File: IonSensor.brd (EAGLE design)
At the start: 50.8 x 22.9 mm, 20 parts, among them IC1 QUAD_OPAMPD, IC2 QUAD_OPAMPD, IC3 QUAD_OPAMPD, X1 JST-XH-04-PIN-LONG-PAD

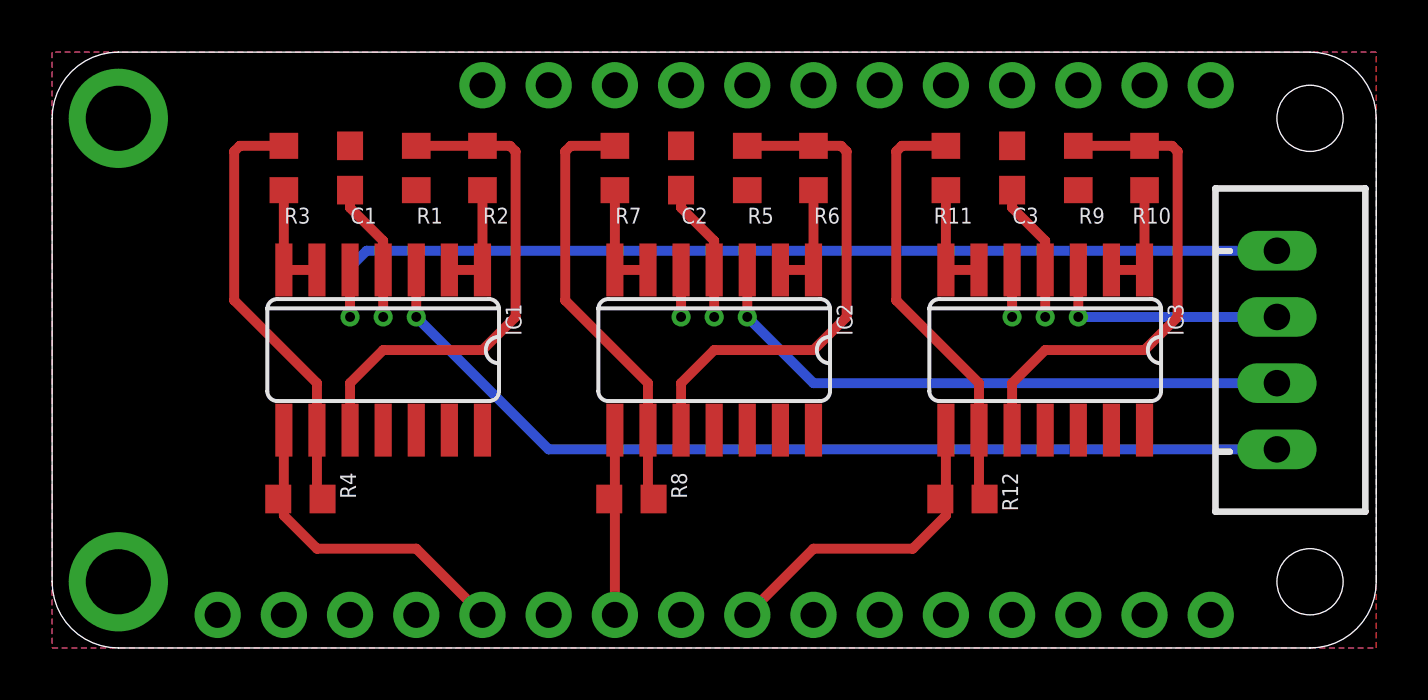
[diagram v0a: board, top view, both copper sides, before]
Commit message: Switch to 2 channel opamp
Switched to 2 channel opamp instead of quad opamp.
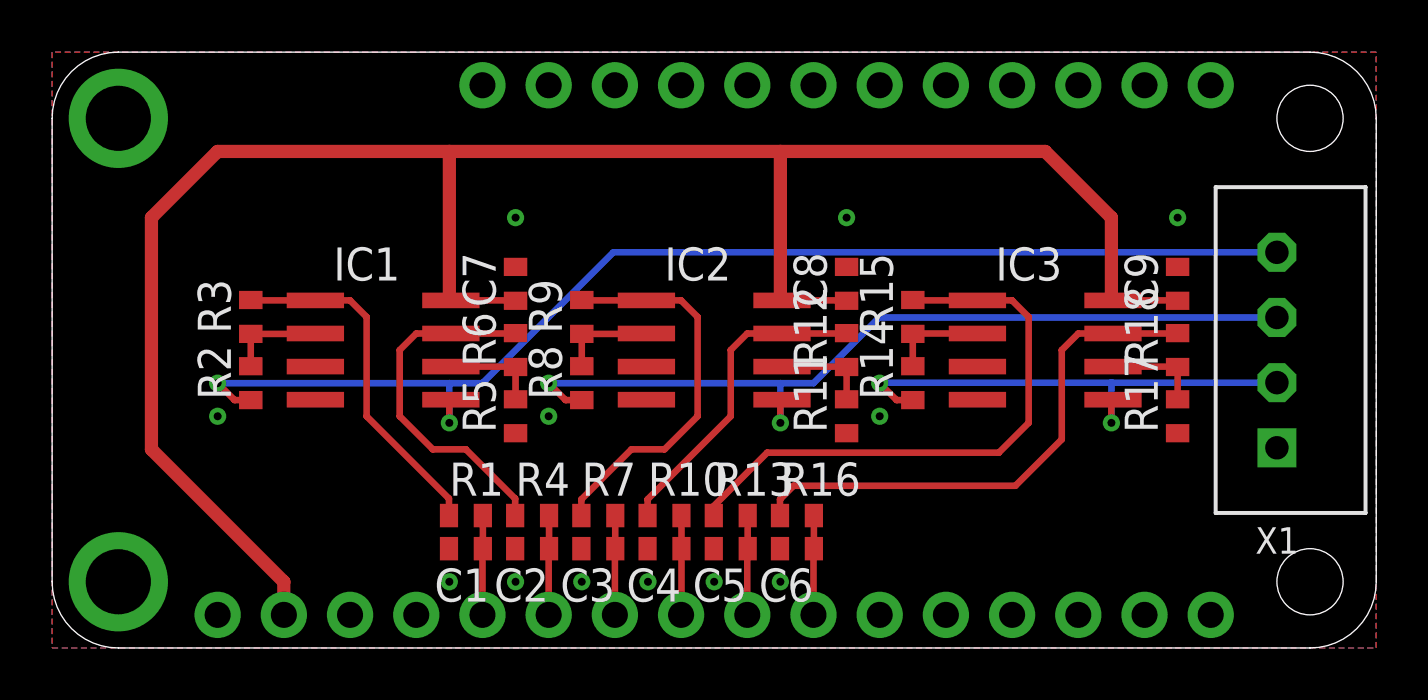
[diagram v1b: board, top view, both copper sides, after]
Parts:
- added C4, C5, C6, C7, C8, C9: 0.1uF, adafruit:C0402
- added R13, R16: 1M, adafruit:R0402
- added R14, R17, R18: 10k, adafruit:R0402
- added R15: 20k, adafruit:R0402
- C1, C2, C3: device adafruit:C0603 -> adafruit:C0402
- IC1, IC2, IC3: value QUAD_OPAMPD -> LM358D; device adafruit:SO14 -> linear:SO08
- R1, R4: value 100k -> 1M; device adafruit:R0603 -> adafruit:R0402
- R10, R7: value 10k -> 1M; device adafruit:R0603 -> adafruit:R0402
- R11, R2, R6: device adafruit:R0603 -> adafruit:R0402
- R12, R5, R8: value 100k -> 10k; device adafruit:R0603 -> adafruit:R0402
- R3: value 10k -> 20k; device adafruit:R0603 -> adafruit:R0402
- R9: value 100k -> 20k; device adafruit:R0603 -> adafruit:R0402
- X1: value JST-XH-04-PIN-LONG-PAD -> B4B-XH-2; device Rembrandt Electronics - JST XH Connectors v1-0:JST-XH-04-PACKAGE-LONG-PAD -> con-JST XH:B4B-XH-A
- moved R10 22.7 mm to (23.5, 5.08), turned to 0 degrees
- moved C3 21.6 mm to (21.0, 3.81), turned to 180 degrees
- moved R9 19.9 mm to (20.3, 12.7)
- moved C2 15.7 mm to (18.4, 3.81), turned to 180 degrees
- moved C1 15.3 mm to (15.9, 3.81), turned to 180 degrees
- moved R1 13.5 mm to (15.9, 5.08), turned to 0 degrees
- moved R6 13.4 mm to (17.8, 11.4)
- moved R7 13.4 mm to (21.0, 5.08), turned to 0 degrees
- moved R5 13.0 mm to (17.8, 8.89)
- moved R2 12.1 mm to (7.62, 10.2)
- moved R11 10.3 mm to (30.5, 8.89)
- moved R4 8.91 mm to (18.4, 5.08), turned to 0 degrees
- moved R12 7.24 mm to (30.5, 11.4), turned to 90 degrees
- moved R3 5.85 mm to (7.62, 12.7)
- moved R8 4.84 mm to (20.3, 10.2), turned to 90 degrees
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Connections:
- removed net N$13: IC3.10, R10.2, R9.2
- removed net N$14: IC3.9, R11.2, R12.1
- removed net REF: IC1.5, IC2.5, IC3.5, X1.1
- new net A1: C2.1, MS1.6, R4.2
- new net A3: C4.1, MS1.8, R10.2
- new net A5: C6.1, MS1.10, R16.2
- new net N$10: IC3.1, R13.1, R15.2
- new net N$5: IC2.2, R8.2, R9.1
- net +3V3: now also C7.1, C8.1, C9.1, IC1.8, IC2.8, IC3.8; no longer C1.1, C2.1, C3.1, IC1.4, IC2.4, IC3.4
- net A0: now also C1.1, R1.2; no longer IC1.8, R4.2
- net A2: now also C3.1, R7.2; no longer IC2.8, R8.2
- net A4: now also C5.1, R13.2; no longer IC3.8, R12.2
- net CH0: now also IC1.5, R2.1; no longer IC1.3
- net CH1: now also IC2.5, R8.1; no longer IC2.3
- net CH2: now also IC3.5, R14.1; no longer IC3.3
- net GND: now also C4.2, C5.2, C6.2, C7.2, C8.2, C9.2, IC1.3, IC1.4, IC2.3, IC2.4, IC3.3, IC3.4, R11.1, R17.1, X1.1; no longer IC1.11, IC2.11, IC3.11, R1.1, R9.1
- net N$1: now also R2.2, R3.1; no longer IC1.1, R2.1
- net N$11: now also IC3.6, R17.2, R18.1; no longer IC3.1, IC3.2, R10.1
- net N$12: now also R16.1, R18.2; no longer IC3.6, R11.1
- net N$2: now also IC1.6, R5.2, R6.1; no longer IC1.10, R1.2, R2.2
- net N$3: now also IC1.1, R1.1, R3.2; no longer IC1.6, IC1.7, R3.1
- net N$4: now also IC1.7, R6.2; no longer IC1.9, R3.2
- net N$6: now also R7.1, R9.2; no longer IC2.2, R6.1
- net N$7: now also R11.2, R12.1; no longer IC2.7, R7.1
- net N$8: now also IC2.7, R10.1, R12.2; no longer IC2.10, R5.2, R6.2
- net N$9: now also IC3.2, R14.2, R15.1; no longer IC2.9, R7.2, R8.1
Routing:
- net +3V3: track 16.2 -> 78.4 mm, vias 3 -> 0
- net REF: track 48.2 -> 0.00 mm, vias 3 -> 0
- net N$10: track 0.00 -> 22.5 mm
- net N$13: track 19.5 -> 0.00 mm
- net N$14: track 16.7 -> 0.00 mm
- net N$12: track 4.33 -> 20.5 mm
- net N$2: track 19.5 -> 3.73 mm
- net N$9: track 16.7 -> 3.73 mm
- net N$6: track 4.33 -> 14.9 mm
- net CH2: track 9.42 -> 19.2 mm, vias 1 -> 2
- net CH1: track 23.2 -> 33.0 mm, vias 1 -> 2
- net CH0: track 36.9 -> 46.7 mm, vias 1 -> 2
- net N$3: track 4.33 -> 13.6 mm
- net A0: track 12.7 -> 3.82 mm
- net A4: track 12.7 -> 3.82 mm
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- added copper zone on layer 16, net GND
- removed copper zone on layer 16, net +3V3
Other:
- board text added: "Rev. D"

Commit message: Revert "Switch to 2 channel opamp"
This reverts commit d2c6276b5e9005aaa4bb267ec01d57cf95291150.
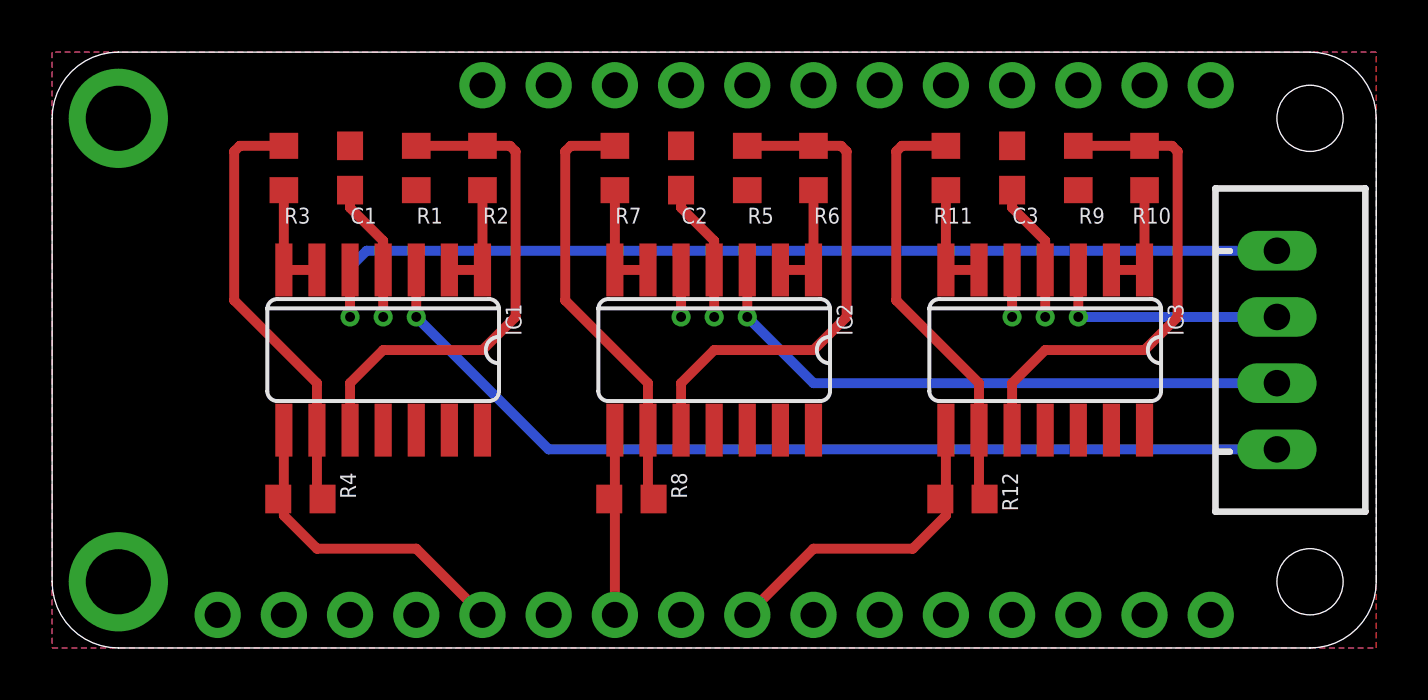
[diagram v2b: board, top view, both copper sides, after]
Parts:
- removed C4, C5, C6, C7, C8, C9: 0.1uF, adafruit:C0402
- removed R13, R16: 1M, adafruit:R0402
- removed R14, R17, R18: 10k, adafruit:R0402
- removed R15: 20k, adafruit:R0402
- C1, C2, C3: device adafruit:C0402 -> adafruit:C0603
- IC1, IC2, IC3: value LM358D -> QUAD_OPAMPD; device linear:SO08 -> adafruit:SO14
- R1, R4: value 1M -> 100k; device adafruit:R0402 -> adafruit:R0603
- R10, R7: value 1M -> 10k; device adafruit:R0402 -> adafruit:R0603
- R11, R2, R6: device adafruit:R0402 -> adafruit:R0603
- R12, R5, R8: value 10k -> 100k; device adafruit:R0402 -> adafruit:R0603
- R3: value 20k -> 10k; device adafruit:R0402 -> adafruit:R0603
- R9: value 20k -> 100k; device adafruit:R0402 -> adafruit:R0603
- X1: value B4B-XH-2 -> JST-XH-04-PIN-LONG-PAD; device con-JST XH:B4B-XH-A -> Rembrandt Electronics - JST XH Connectors v1-0:JST-XH-04-PACKAGE-LONG-PAD
- moved R10 22.7 mm to (41.9, 18.4), turned to 90 degrees
- moved C3 21.6 mm to (36.8, 18.4), turned to 90 degrees
- moved R9 19.9 mm to (39.4, 18.4)
- moved C2 15.7 mm to (24.1, 18.4), turned to 90 degrees
- moved C1 15.3 mm to (11.4, 18.4), turned to 90 degrees
- moved R1 13.5 mm to (14.0, 18.4), turned to 90 degrees
- moved R6 13.4 mm to (29.2, 18.4)
- moved R7 13.4 mm to (21.6, 18.4), turned to 90 degrees
- moved R5 13.0 mm to (26.7, 18.4)
- moved R2 12.1 mm to (16.5, 18.4)
- moved R11 10.3 mm to (34.3, 18.4)
- moved R4 8.91 mm to (9.53, 5.71), turned to 180 degrees
- moved R12 7.24 mm to (34.9, 5.71), turned to 180 degrees
- moved R3 5.85 mm to (8.89, 18.4)
- moved R8 4.84 mm to (22.2, 5.71), turned to 180 degrees
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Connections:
- removed net A1: C2.1, MS1.6, R4.2
- removed net A3: C4.1, MS1.8, R10.2
- removed net A5: C6.1, MS1.10, R16.2
- removed net N$10: IC3.1, R13.1, R15.2
- removed net N$5: IC2.2, R8.2, R9.1
- new net N$13: IC3.10, R10.2, R9.2
- new net N$14: IC3.9, R11.2, R12.1
- new net REF: IC1.5, IC2.5, IC3.5, X1.1
- net +3V3: now also C1.1, C2.1, C3.1, IC1.4, IC2.4, IC3.4; no longer C7.1, C8.1, C9.1, IC1.8, IC2.8, IC3.8
- net A0: now also IC1.8, R4.2; no longer C1.1, R1.2
- net A2: now also IC2.8, R8.2; no longer C3.1, R7.2
- net A4: now also IC3.8, R12.2; no longer C5.1, R13.2
- net CH0: now also IC1.3; no longer IC1.5, R2.1
- net CH1: now also IC2.3; no longer IC2.5, R8.1
- net CH2: now also IC3.3; no longer IC3.5, R14.1
- net GND: now also IC1.11, IC2.11, IC3.11, R1.1, R9.1; no longer C4.2, C5.2, C6.2, C7.2, C8.2, C9.2, IC1.3, IC1.4, IC2.3, IC2.4, IC3.3, IC3.4, R11.1, R17.1, X1.1
- net N$1: now also IC1.1, R2.1; no longer R2.2, R3.1
- net N$11: now also IC3.1, IC3.2, R10.1; no longer IC3.6, R17.2, R18.1
- net N$12: now also IC3.6, R11.1; no longer R16.1, R18.2
- net N$2: now also IC1.10, R1.2, R2.2; no longer IC1.6, R5.2, R6.1
- net N$3: now also IC1.6, IC1.7, R3.1; no longer IC1.1, R1.1, R3.2
- net N$4: now also IC1.9, R3.2; no longer IC1.7, R6.2
- net N$6: now also IC2.2, R6.1; no longer R7.1, R9.2
- net N$7: now also IC2.7, R7.1; no longer R11.2, R12.1
- net N$8: now also IC2.10, R5.2, R6.2; no longer IC2.7, R10.1, R12.2
- net N$9: now also IC2.9, R7.2, R8.1; no longer IC3.2, R14.2, R15.1
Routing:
- net +3V3: track 78.4 -> 16.2 mm, vias 0 -> 3
- net REF: track 0.00 -> 48.2 mm, vias 0 -> 3
- net N$10: track 22.5 -> 0.00 mm
- net N$13: track 0.00 -> 19.5 mm
- net N$14: track 0.00 -> 16.7 mm
- net N$12: track 20.5 -> 4.33 mm
- net N$2: track 3.73 -> 19.5 mm
- net N$9: track 3.73 -> 16.7 mm
- net N$6: track 14.9 -> 4.33 mm
- net CH2: track 19.2 -> 9.42 mm, vias 2 -> 1
- net CH1: track 33.0 -> 23.2 mm, vias 2 -> 1
- net CH0: track 46.7 -> 36.9 mm, vias 2 -> 1
- net N$3: track 13.6 -> 4.33 mm
- net A0: track 3.82 -> 12.7 mm
- net A4: track 3.82 -> 12.7 mm
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- added copper zone on layer 16, net +3V3
- removed copper zone on layer 16, net GND
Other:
- board text removed: "Rev. D"

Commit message: Rev. D
Upgrade to Rev. D, no connector
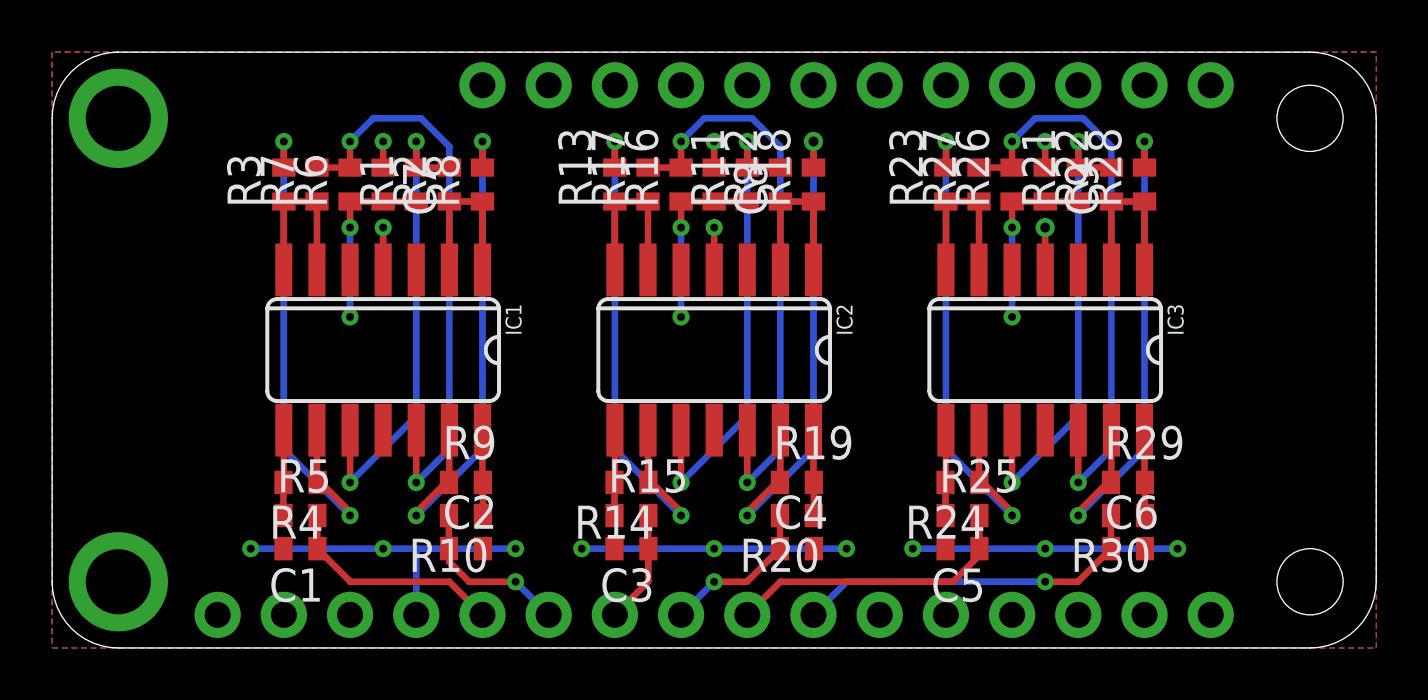
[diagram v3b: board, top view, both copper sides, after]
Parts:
- removed X1: JST-XH-04-PIN-LONG-PAD, Rembrandt Electronics - JST XH Connectors v1-0:JST-XH-04-PACKAGE-LONG-PAD
- added C4, C5, C6, C7, C8, C9: 0.1uF, adafruit:C0402
- added R13, R17, R18, R22, R23, R27, R28: 10k, adafruit:R0402
- added R14, R16, R19, R21, R24, R26, R29: 100k, adafruit:R0402
- added R15, R20, R25, R30: 1M, adafruit:R0402
- C1, C2, C3: device adafruit:C0603 -> adafruit:C0402
- R1, R2, R3, R4, R7, R9: device adafruit:R0603 -> adafruit:R0402
- R10: value 10k -> 1M; device adafruit:R0603 -> adafruit:R0402
- R11, R6: value 10k -> 100k; device adafruit:R0603 -> adafruit:R0402
- R12, R8: value 100k -> 10k; device adafruit:R0603 -> adafruit:R0402
- R5: value 100k -> 1M; device adafruit:R0603 -> adafruit:R0402
- moved R10 29.3 mm to (15.9, 5.08), turned to 180 degrees
- moved R9 26.4 mm to (15.9, 6.35), turned to 0 degrees
- moved R5 21.7 mm to (9.53, 5.08), turned to 0 degrees
- moved C3 20.7 mm to (22.2, 3.81), turned to 180 degrees
- moved R6 17.8 mm to (11.4, 17.8)
- moved C2 16.8 mm to (15.9, 3.81), turned to 0 degrees
- moved C1 14.7 mm to (9.53, 3.81), turned to 180 degrees
- moved R12 13.9 mm to (27.9, 17.8), turned to 90 degrees
- moved R8 13.4 mm to (16.5, 17.8), turned to 90 degrees
- moved R7 11.4 mm to (10.2, 17.8)
- moved R11 7.65 mm to (26.7, 17.8)
- moved R2 1.42 mm to (15.2, 17.8)
- moved R4 0.63 mm to (9.53, 6.35)
- moved R1 0.63 mm to (14.0, 17.8)
- moved R3 0.63 mm to (8.89, 17.8)
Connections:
- removed net N$1 (its old number): IC1.1, IC1.2, R2.1
- new net A1: C2.1, MS1.6, R10.2
- new net A3: C4.1, MS1.8, R20.2
- new net A5: C6.1, MS1.10, R30.2
- new net C1+: IC1.1, IC1.2, R2.1, R8.1
- new net C1-: IC1.6, IC1.7, R3.1, R7.1
- new net C2+: IC2.1, IC2.2, R12.1, R18.1
- new net C2-: IC2.6, IC2.7, R13.1, R17.1
- new net C3+: IC3.1, IC3.2, R22.1, R28.1
- new net C3-: IC3.6, IC3.7, R23.1, R27.1
- new net N$10: IC1.14, R10.1, R9.2
- new net N$15: IC3.13, R28.2, R29.1
- new net N$16: IC2.14, R19.2, R20.1
- new net N$17: IC3.8, R24.2, R25.1
- new net N$18: IC3.14, R29.2, R30.1
- new net N$4: IC1.12, R6.2, R7.2
- new net N$5: IC1.8, R4.2, R5.1
- net +3V3: now also C7.1, C8.1, C9.1; no longer C1.1, C2.1, C3.1
- net A0: now also C1.1, R5.2; no longer IC1.8, R4.2
- net A2: now also C3.1, R15.2; no longer IC2.8, R8.2
- net A4: now also C5.1, R25.2; no longer IC3.8, R12.2
- net CH0: no longer X1.4
- net CH1: no longer X1.3
- net CH2: no longer X1.2
- net GND: now also C4.2, C5.2, C6.2, C7.2, C8.2, C9.2, R11.1, R16.1, R21.1, R26.1, R6.1; no longer R5.1, R9.1
- net N$11: now also IC2.12, R16.2, R17.2; no longer IC3.1, IC3.2, R10.1
- net N$12: now also IC3.12, R26.2, R27.2; no longer IC3.6, IC3.7, R11.1
- net N$13: now also IC2.13, R18.2, R19.1; no longer IC3.10, R10.2, R9.2
- net N$14: now also IC2.8, R14.2, R15.1; no longer IC3.9, R11.2, R12.1
- net N$3: now also IC3.10, R21.2, R22.2; no longer IC1.6, IC1.7, R3.1
- net N$6: now also IC1.13, R8.2, R9.1; no longer IC2.1, IC2.2, R6.1
- net N$7: now also IC3.9, R23.2, R24.1; no longer IC2.6, IC2.7, R7.1
- net N$8: now also R11.2, R12.2; no longer R5.2, R6.2
- net N$9: now also R13.2, R14.1; no longer R7.2, R8.1
- net REF: no longer X1.1
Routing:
- net GND: track 0.00 -> 53.9 mm, vias 0 -> 15
- net REF: track 48.2 -> 0.00 mm, vias 3 -> 0
- net CH0: track 36.9 -> 0.00 mm, vias 1 -> 0
- net CH1: track 23.2 -> 0.00 mm, vias 1 -> 0
- net N$4: track 0.00 -> 22.3 mm, vias 0 -> 2
- net N$15: track 0.00 -> 20.3 mm, vias 0 -> 2
- net N$11: track 4.33 -> 22.3 mm, vias 0 -> 2
- net N$12: track 4.33 -> 22.3 mm, vias 0 -> 2
- net N$7: track 4.33 -> 20.3 mm, vias 0 -> 2
- net N$6: track 4.33 -> 20.3 mm, vias 0 -> 2
- net N$3: track 4.33 -> 18.4 mm, vias 0 -> 2
- net A5: track 0.00 -> 13.7 mm, vias 0 -> 1
- net N$14: track 16.7 -> 3.28 mm
- net CH2: track 9.42 -> 0.00 mm, vias 1 -> 0
- net +3V3: track 16.2 -> 7.88 mm, vias 3 -> 6
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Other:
- board text added: "Rev. D"
